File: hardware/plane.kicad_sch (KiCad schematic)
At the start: 21 parts, among them J1 USB_B_Micro, Q1 BSS138, Q2 BSS138, U1 ESP32-WROOM-32, U2 AMS1117-3.3, U3 CH340C

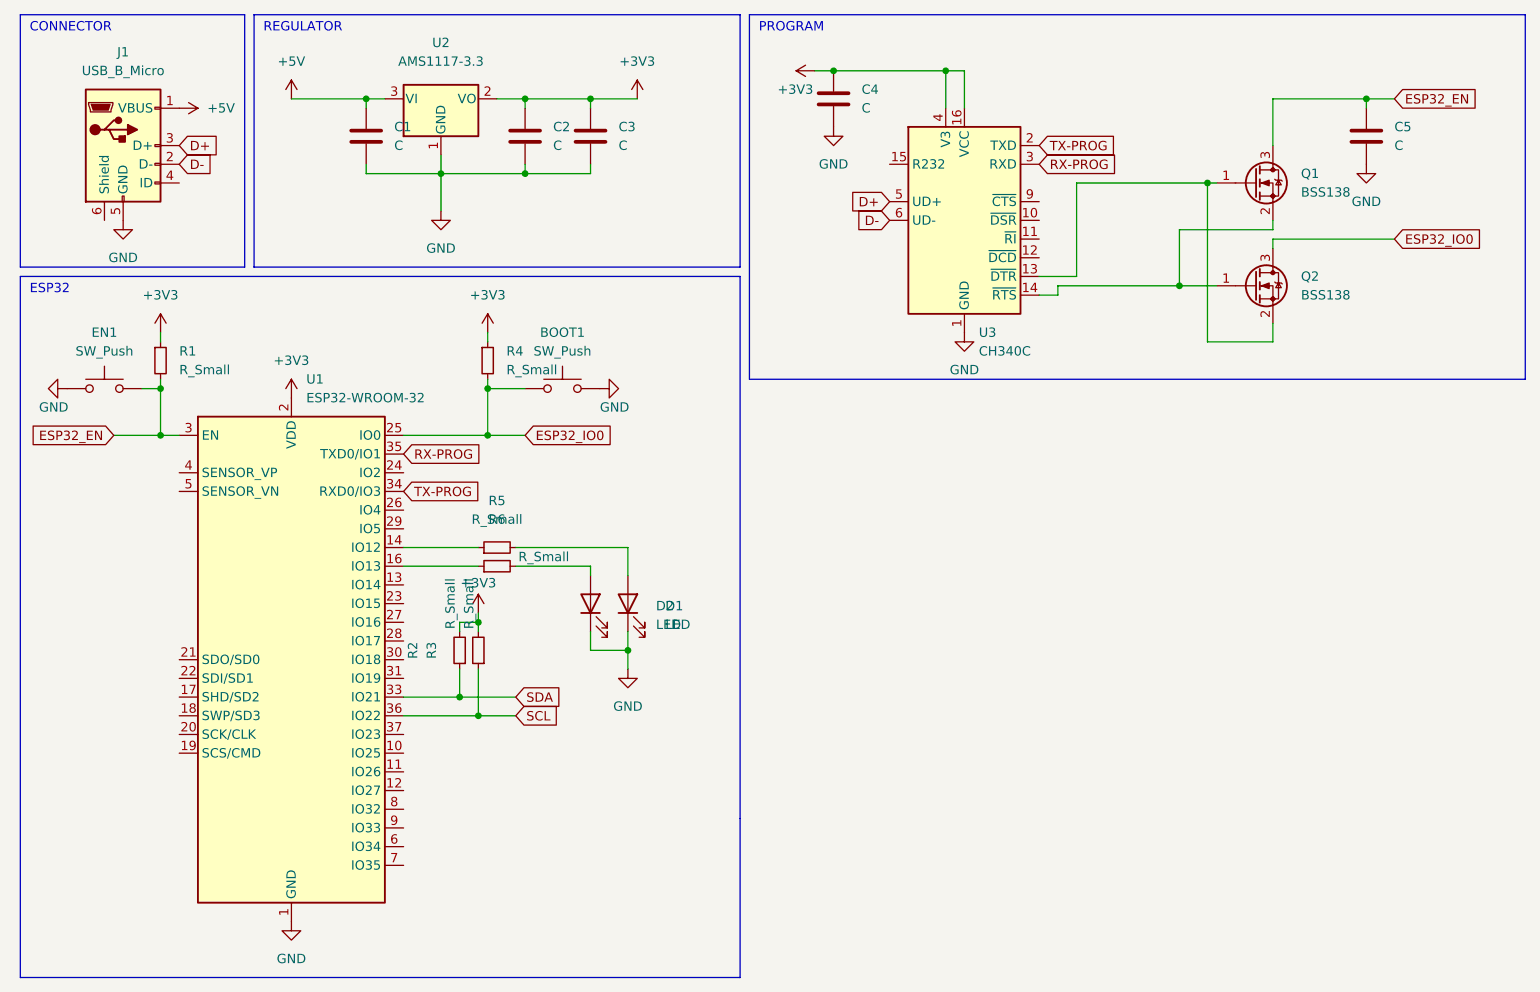
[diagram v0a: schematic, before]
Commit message: add lora
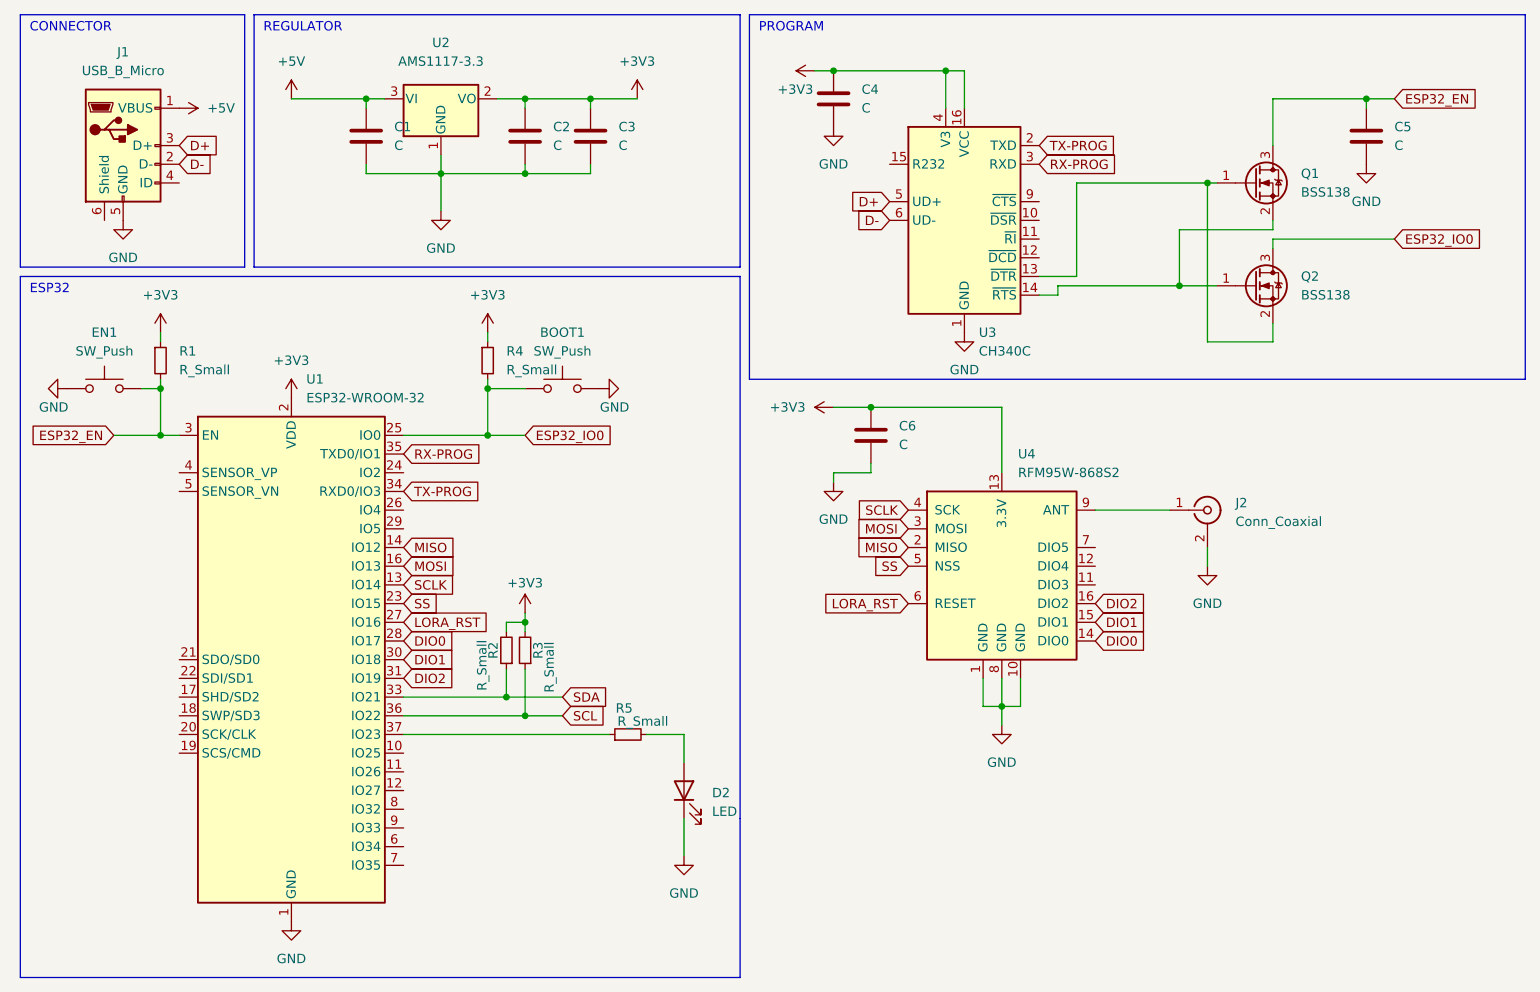
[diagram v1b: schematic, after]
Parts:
- removed D1: LED, LED_SMD:LED_0603_1608Metric, symbol Device:LED
- removed R6: R_Small, Resistor_SMD:R_0603_1608Metric, symbol Device:R_Small
- added C6: C, Capacitor_SMD:C_0603_1608Metric, symbol Device:C
- added J2: Conn_Coaxial, symbol Connector:Conn_Coaxial
- added U4: RFM95W-868S2, symbol RF_Module:RFM95W-868S2
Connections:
- net +3V3: now also C6.1, U4.13 (3.3V)
- net GND: now also C6.2, J2.2 (Ext), U4.1 (GND), U4.10 (GND), U4.8 (GND)
- net MOSI: now reaches U1.16 (IO13)
- net MOSI: now also U4.3 (MOSI)
- net SCLK: now reaches U1.13 (IO14)
- net SCLK: now also U4.4 (SCK)
- net at R5.1: now also U1.37 (IO23); no longer U1.14 (IO12)
- net SS: now reaches U1.23 (IO15)
- net SS: now also U4.5 (NSS)
- net LORA_RST: now reaches U1.27 (IO16)
- net LORA_RST: now also U4.6 (RESET)
- net DIO0: now reaches U1.28 (IO17)
- net DIO0: now also U4.14 (DIO0)
- net DIO1: now reaches U1.30 (IO18)
- net DIO1: now also U4.15 (DIO1)
- net DIO2: now reaches U1.31 (IO19)
- net DIO2: now also U4.16 (DIO2)
- new net: J2.1 (In), U4.9 (ANT)
- new net MISO: U1.14 (IO12), U4.2 (MISO)
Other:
- moved on the sheet: D2, R2, R3, R5
